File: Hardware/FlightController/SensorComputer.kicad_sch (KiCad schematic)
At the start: 0 parts

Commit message: Add Sensor MCU schematic items
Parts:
- added C10, C12: 2.2uF, Capacitor_SMD:C_0603_1608Metric, symbol Device:C_Small
- added C11, C13, C14, C15, C9: 100nF, Capacitor_SMD:C_0603_1608Metric, symbol Device:C_Small
- added C16: 1uF, Capacitor_SMD:C_0603_1608Metric, symbol Device:C_Small
- added C17: 10nF, Capacitor_SMD:C_0603_1608Metric, symbol Device:C_Small
- added C6, C7: 12pF, Capacitor_SMD:C_0603_1608Metric, symbol Device:C_Small
- added C8: 4.7uF, Capacitor_SMD:C_0603_1608Metric, symbol Device:C_Small
- added J2: USB_B_Mini, symbol Connector:USB_B_Mini
- added J3: Conn_01x04, symbol Connector_Generic:Conn_01x04
- added J4: Conn_02x03_Odd_Even, symbol Connector_Generic:Conn_02x03_Odd_Even
- added L2: 39nH, Inductor_SMD:L_0402_1005Metric, symbol Device:L_Small
- added R3: 10k, Resistor_SMD:R_0603_1608Metric, symbol Device:R_Small
- added R4: 47, Resistor_SMD:R_0603_1608Metric, symbol Device:R_Small
- added R5, R6: 2.2k, Resistor_SMD:R_0603_1608Metric, symbol Device:R_Small
- added SW1: SW_SPDT, symbol Switch:SW_SPDT
- added U1: STM32F405RGT6, Package_QFP:LQFP-64_10x10mm_P0.5mm, symbol MCU_ST_STM32F4:STM32F405RGTx
- added Y1: 16MHz, Crystal:Crystal_SMD_3225-4Pin_3.2x2.5mm, symbol Device:Crystal_GND24
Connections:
- new net: C12.1, U1.47 (VCAP_2)
- new net: R3.2, SW1.2 (B)
- new net: C7.1, R4.2, Y1.3
- new net: C10.1, U1.31 (VCAP_1)
- new net +3.3VA: C16.1, C17.1, L2.2, U1.13 (VDDA)
- new net +3V3: C11.1, C13.1, C14.1, C15.1, C8.1, C9.1, J3.1 (Pin_1), J4.1 (Pin_1), L2.1, R5.2, R6.2, SW1.1 (A), U1.1 (VBAT), U1.19 (VDD), U1.32 (VDD), U1.48 (VDD), U1.64 (VDD)
- new net +5V: J2.1 (VBUS)
- new net CAN_RX: U1.61 (PB8)
- new net CAN_TX: U1.62 (PB9)
- new net GND: C10.2, C11.2, C12.2, C13.2, C14.2, C15.2, C16.2, C17.2, C6.2, C7.2, C8.2, C9.2, J2.5 (GND), J3.4 (Pin_4), J4.3 (Pin_3), SW1.3 (C), U1.12 (VSSA), U1.18 (VSS), U1.63 (VSS), Y1.2, Y1.4
- new net S_BOOT0: R3.1, U1.60 (BOOT0)
- new net S_HSE_IN: C6.1, U1.5 (PH0), Y1.1
- new net S_HSE_OUT: R4.1, U1.6 (PH1)
- new net S_I2C1_SCL: R5.1, U1.58 (PB6)
- new net S_I2C1_SDA: R6.1, U1.59 (PB7)
- new net S_NRST: J4.5 (Pin_5), U1.7 (NRST)
- new net S_SWCLK: J4.4 (Pin_4), U1.49 (PA14)
- new net S_SWDIO: J4.2 (Pin_2), U1.46 (PA13)
- new net S_SWO: J4.6 (Pin_6), U1.55 (PB3)
- new net S_USART2_RX: U1.17 (PA3)
- new net S_USART2_TX: U1.16 (PA2)
- new net S_USART3_RX: J3.2 (Pin_2), U1.30 (PB11)
- new net S_USART3_TX: J3.3 (Pin_3), U1.29 (PB10)
- new net S_USB_DM: J2.2 (D-), U1.44 (PA11)
- new net S_USB_DP: J2.3 (D+), U1.45 (PA12)
- no-connect marks 0 -> 38
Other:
- note added: "Boot Switch"
- note added: "Clock"
- note added: "Decoupling"

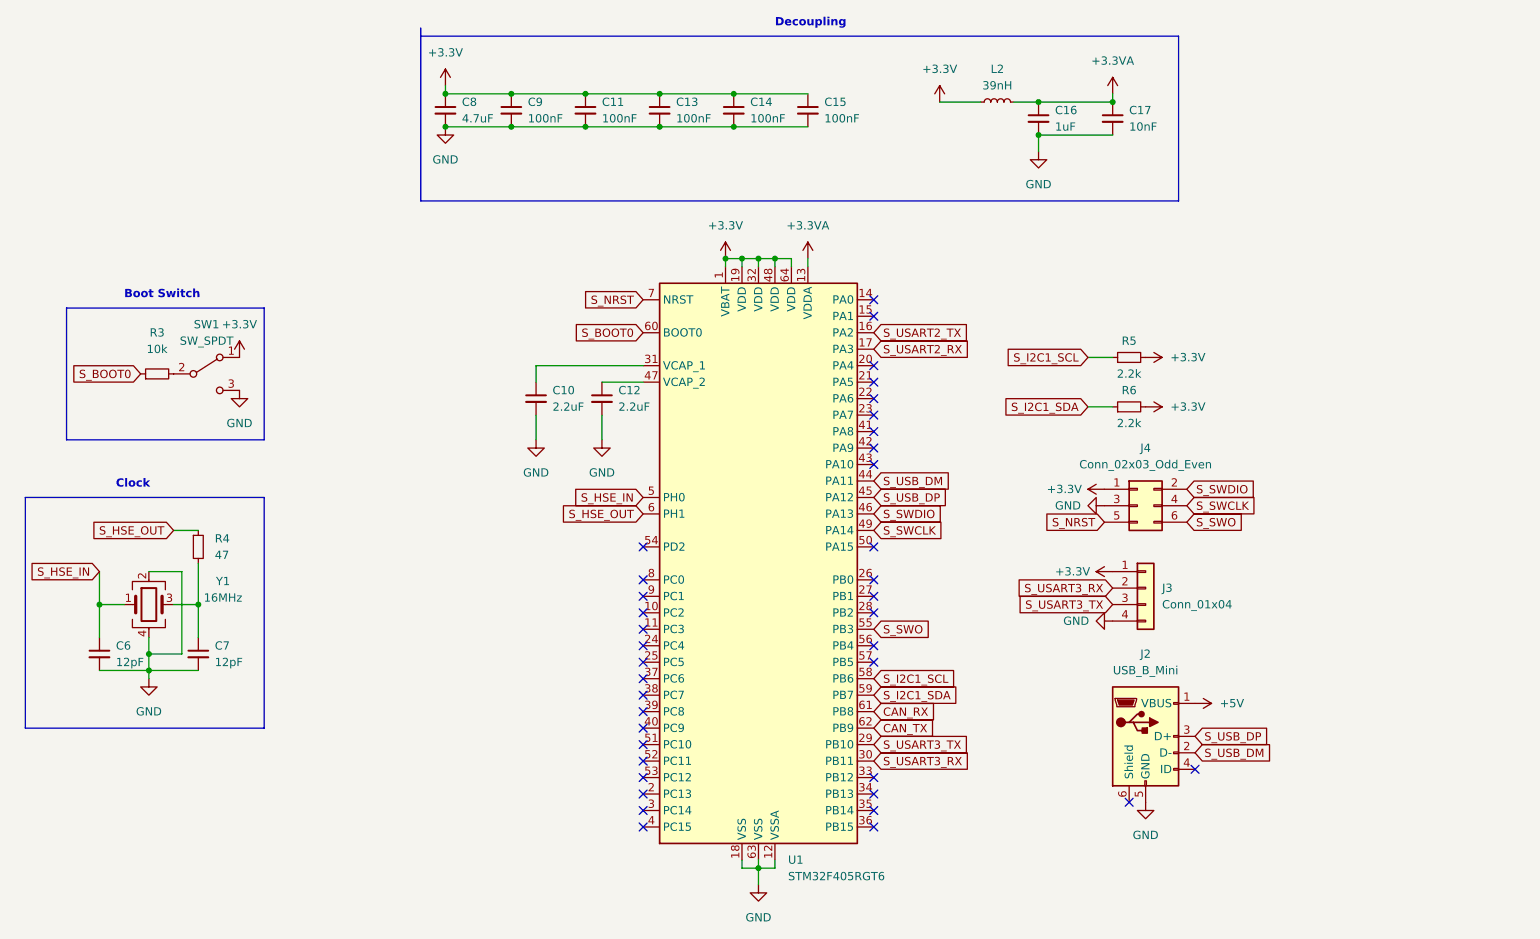
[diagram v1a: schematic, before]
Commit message: Add ICM-42670-P symbol and schematic
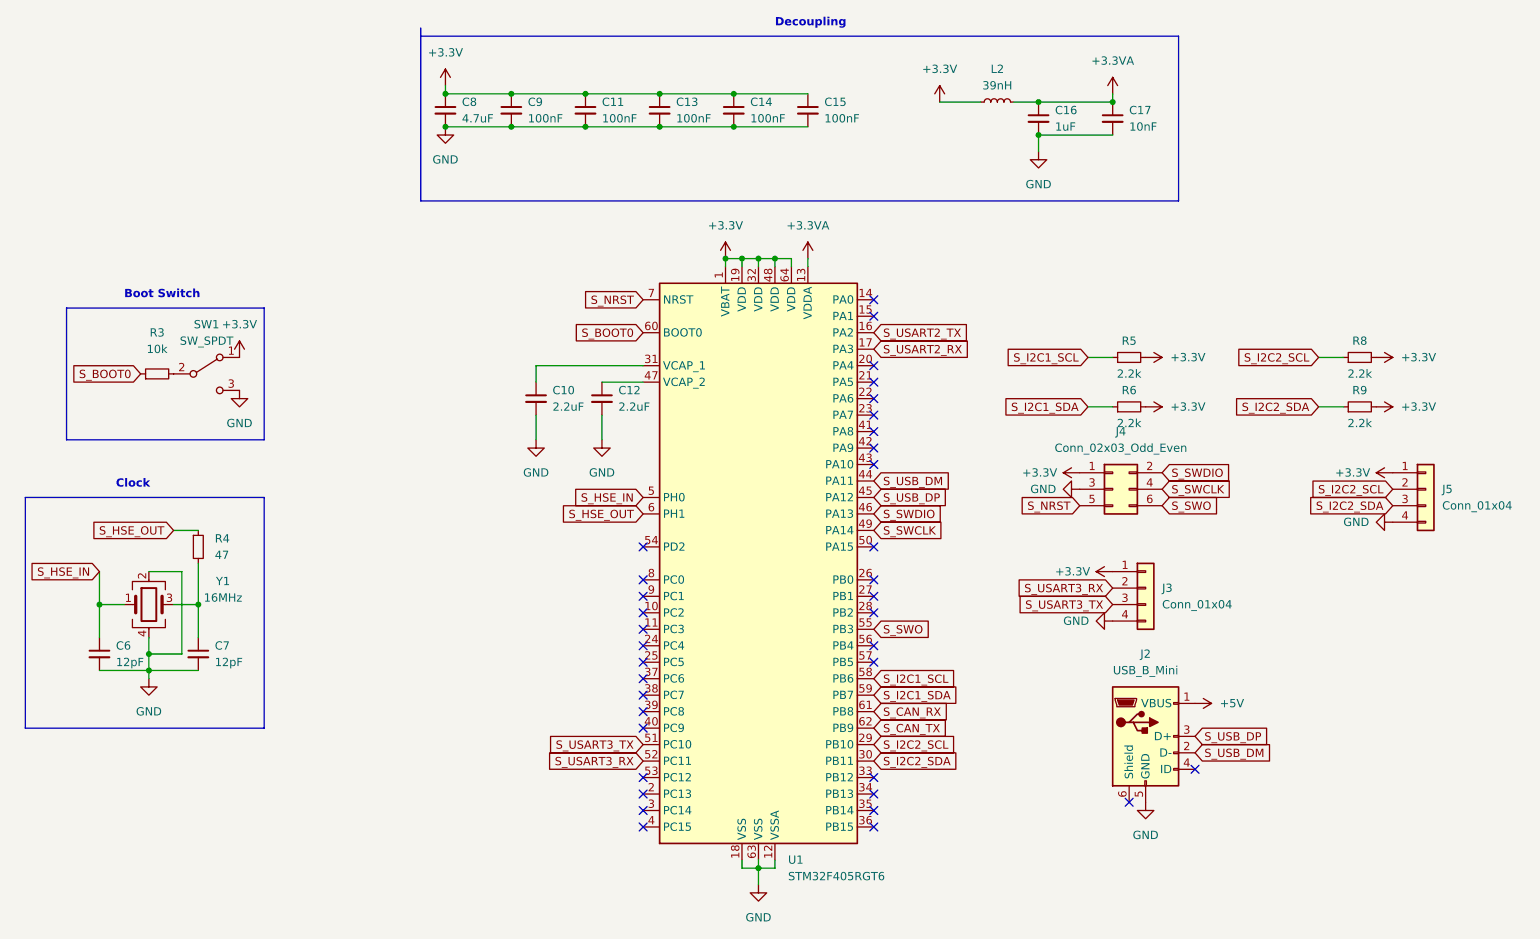
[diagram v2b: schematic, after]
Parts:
- added J5: Conn_01x04, symbol Connector_Generic:Conn_01x04
- added R8, R9: 2.2k, Resistor_SMD:R_0603_1608Metric, symbol Device:R_Small
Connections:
- net +3V3: now also J5.1 (Pin_1), R8.2, R9.2
- net GND: now also J5.4 (Pin_4)
- net S_USART3_RX: now also U1.52 (PC11); no longer U1.30 (PB11)
- net S_USART3_TX: now also U1.51 (PC10); no longer U1.29 (PB10)
- net CAN_RX renamed S_CAN_RX
- net CAN_TX renamed S_CAN_TX
- new net S_I2C2_SCL: J5.2 (Pin_2), R8.1, U1.29 (PB10)
- new net S_I2C2_SDA: J5.3 (Pin_3), R9.1, U1.30 (PB11)
- no-connect marks 38 -> 36
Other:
- moved on the sheet: J4
